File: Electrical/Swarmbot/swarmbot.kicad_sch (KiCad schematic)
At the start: 5 parts, among them J1 Conn_02x07_Counter_Clockwise, J2 Conn_02x07_Counter_Clockwise

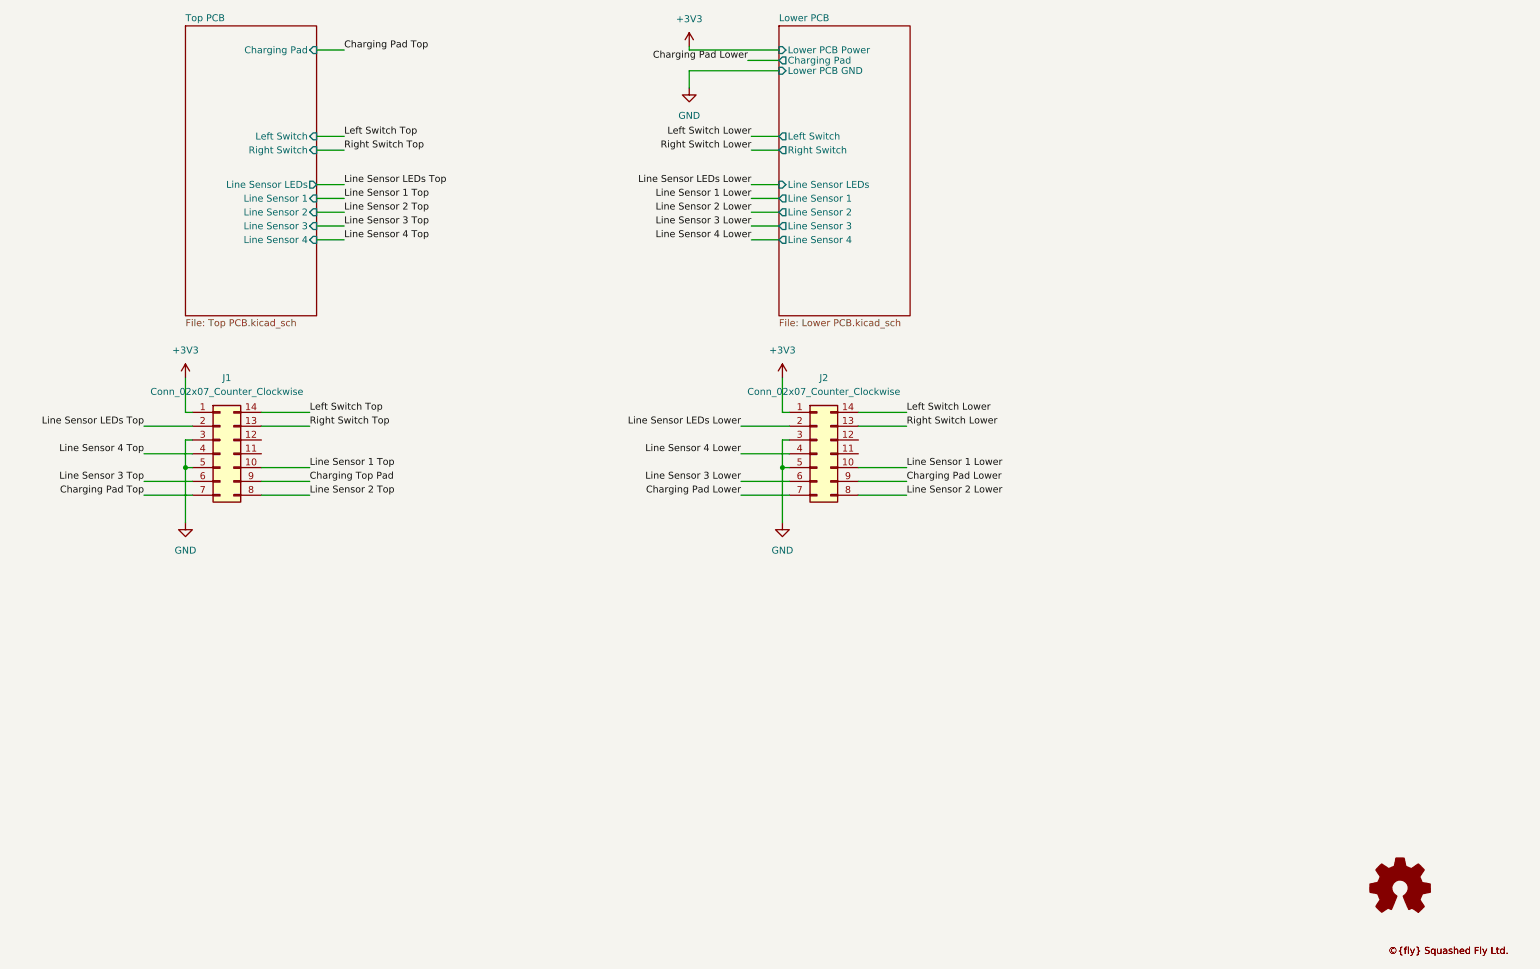
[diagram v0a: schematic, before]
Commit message: some little changes have been made
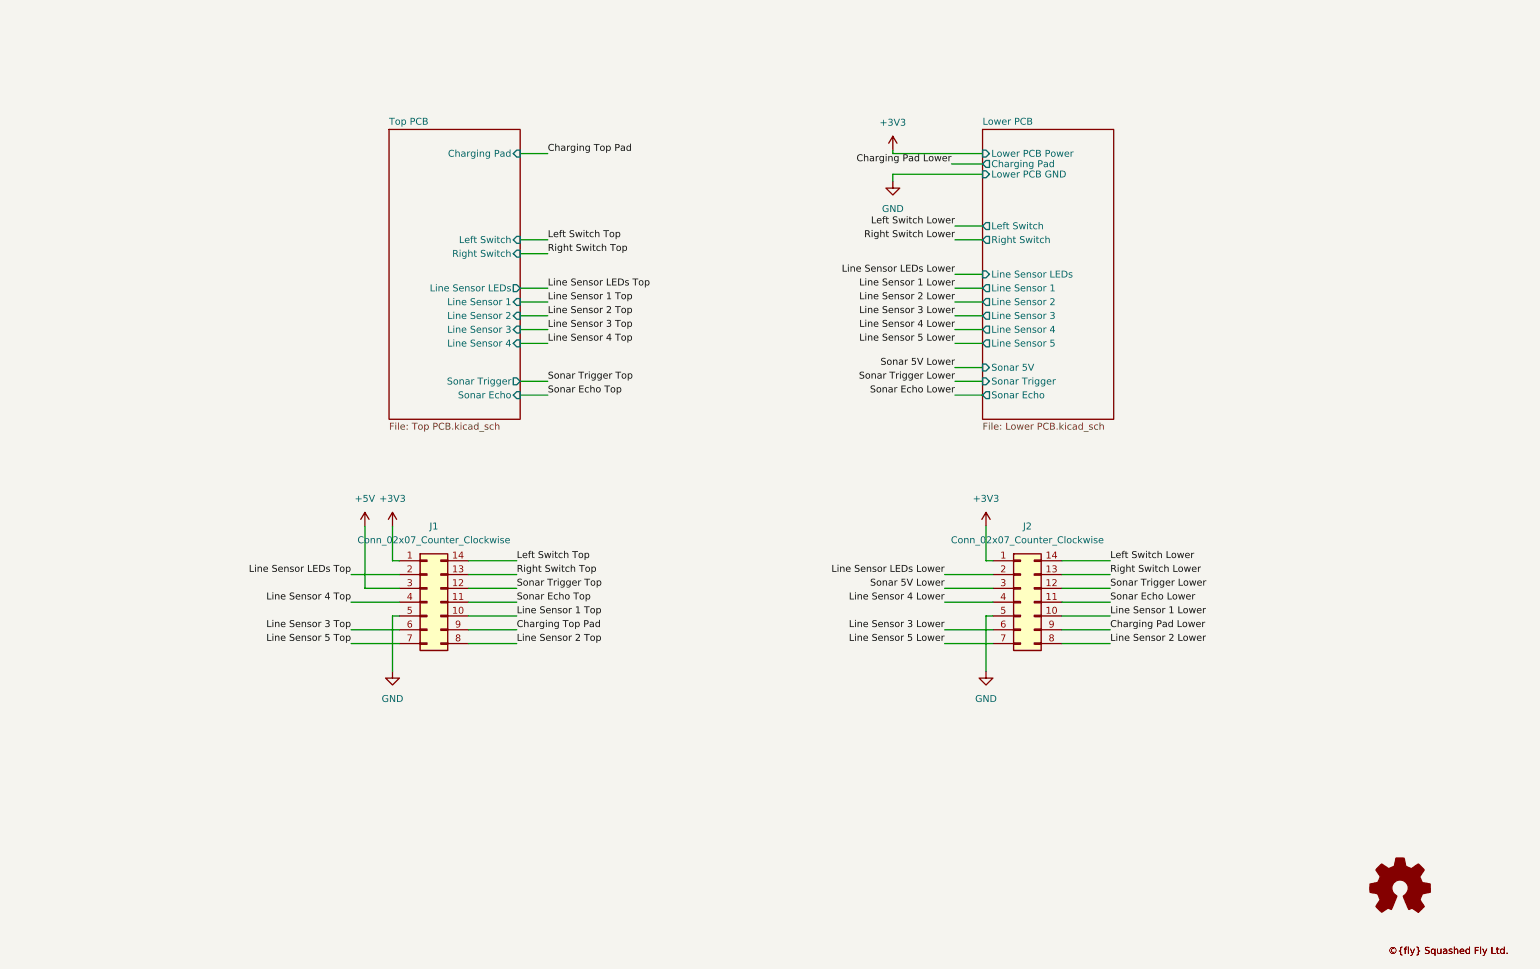
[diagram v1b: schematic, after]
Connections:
- net Charging Pad Lower: no longer J2.7 (Pin_7)
- net GND: no longer J1.3 (Pin_3), J2.3 (Pin_3)
- net Sonar Echo Top: now reaches J1.11 (Pin_11)
- net Sonar Trigger Top: now reaches J1.12 (Pin_12)
- net Sonar Echo Lower: now reaches J2.11 (Pin_11)
- net Sonar Trigger Lower: now reaches J2.12 (Pin_12)
- net Charging Pad Top renamed Line Sensor 5 Top
- new net +5V: J1.3 (Pin_3)
- new net Line Sensor 5 Lower: J2.7 (Pin_7)
- new net Sonar 5V Lower: J2.3 (Pin_3)
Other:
- sheet Lower PCB ports: added Line Sensor 5, Sonar 5V, Sonar Echo, Sonar Trigger; removed none
- sheet Top PCB ports: added Sonar Echo, Sonar Trigger; removed none
- moved on the sheet: J1, J2

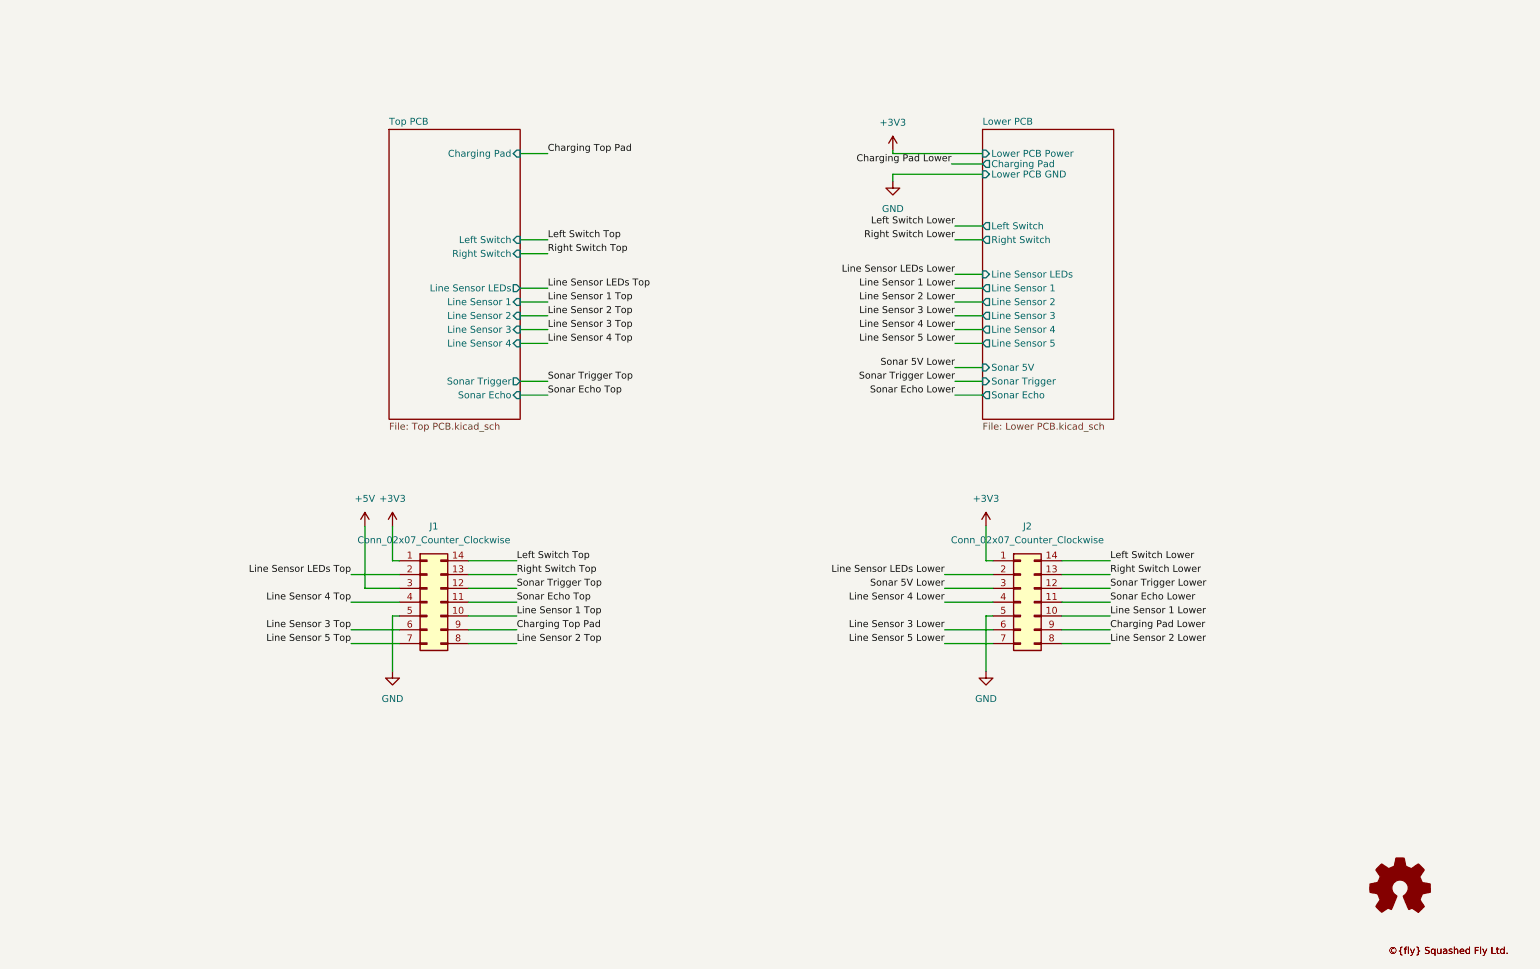
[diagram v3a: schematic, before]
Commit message: Made some Changes
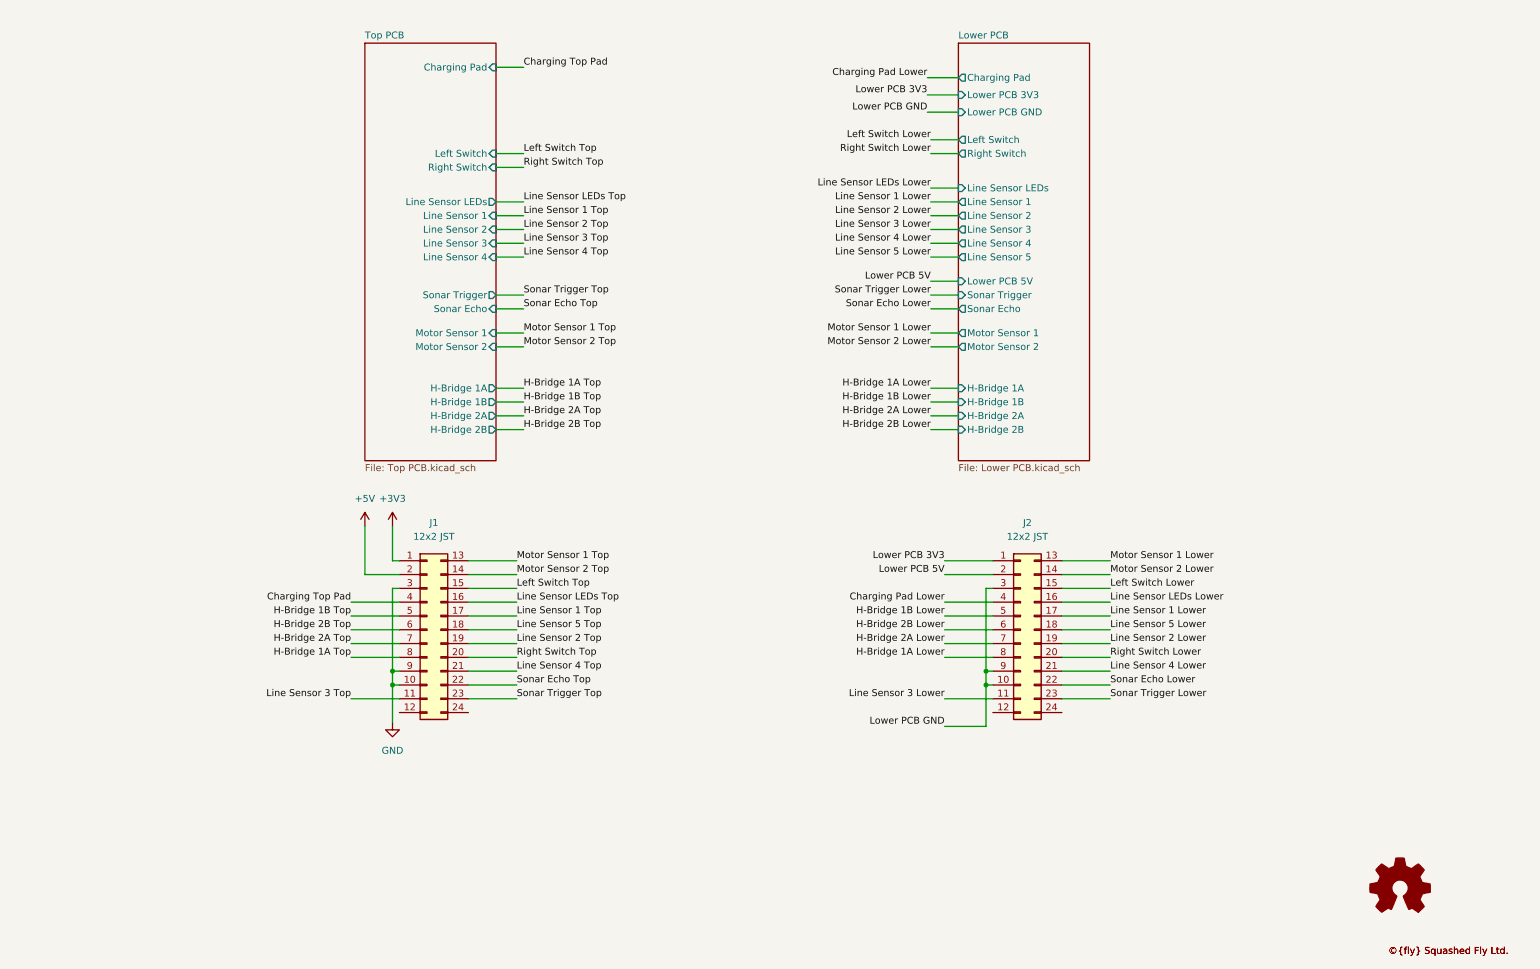
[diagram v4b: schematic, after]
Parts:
- removed J1, J2: Conn_02x07_Counter_Clockwise, Connector_JST:JST_PUD_B14B-PUDSS_2x07_P2.00mm_Vertical, symbol Connector_Generic:Conn_02x07_Counter_Clockwise
- added J1, J2: 12x2 JST, Connector_JST:JST_PUD_B24B-PUDSS_2x12_P2.00mm_Vertical, symbol Connector_Generic:Conn_02x12_Top_Bottom
- Logo2: footprint SquashedFly Logo:SquashedFlyBrightCopper -> SquashedFly Logo:SquashedFlySilk
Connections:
- net +3V3: now also J1.1 (Pin_1)
- net +5V: now also J1.2 (Pin_2)
- net Charging Pad Lower: now also J2.4 (Pin_4)
- net Charging Top Pad: now also J1.4 (Pin_4)
- net GND: now also J1.10 (Pin_10), J1.3 (Pin_3), J1.9 (Pin_9)
- net Left Switch Lower: now also J2.15 (Pin_15)
- net Left Switch Top: now also J1.15 (Pin_15)
- net Line Sensor 1 Lower: now also J2.17 (Pin_17)
- net Line Sensor 1 Top: now also J1.17 (Pin_17)
- net Line Sensor 2 Lower: now also J2.19 (Pin_19)
- net Line Sensor 2 Top: now also J1.19 (Pin_19)
- net Line Sensor 3 Lower: now also J2.11 (Pin_11)
- net Line Sensor 3 Top: now also J1.11 (Pin_11)
- net Line Sensor 4 Lower: now also J2.21 (Pin_21)
- net Line Sensor 4 Top: now also J1.21 (Pin_21)
- net Line Sensor 5 Lower: now also J2.18 (Pin_18)
- net Line Sensor 5 Top: now also J1.18 (Pin_18)
- net Line Sensor LEDs Lower: now also J2.16 (Pin_16)
- net Line Sensor LEDs Top: now also J1.16 (Pin_16)
- net Right Switch Lower: now also J2.20 (Pin_20)
- net Right Switch Top: now also J1.20 (Pin_20)
- net Sonar Echo Lower: now also J2.22 (Pin_22)
- net Sonar Echo Top: now also J1.22 (Pin_22)
- net Sonar Trigger Lower: now also J2.23 (Pin_23)
- net Sonar Trigger Top: now also J1.23 (Pin_23)
- new net H-Bridge 1A Lower: J2.8 (Pin_8)
- new net H-Bridge 1A Top: J1.8 (Pin_8)
- new net H-Bridge 1B Lower: J2.5 (Pin_5)
- new net H-Bridge 1B Top: J1.5 (Pin_5)
- new net H-Bridge 2A Lower: J2.7 (Pin_7)
- new net H-Bridge 2A Top: J1.7 (Pin_7)
- new net H-Bridge 2B Lower: J2.6 (Pin_6)
- new net H-Bridge 2B Top: J1.6 (Pin_6)
- new net Lower PCB 3V3: J2.1 (Pin_1)
- new net Lower PCB 5V: J2.2 (Pin_2)
- new net Lower PCB GND: J2.10 (Pin_10), J2.3 (Pin_3), J2.9 (Pin_9)
- new net Motor Sensor 1 Lower: J2.13 (Pin_13)
- new net Motor Sensor 1 Top: J1.13 (Pin_13)
- new net Motor Sensor 2 Lower: J2.14 (Pin_14)
- new net Motor Sensor 2 Top: J1.14 (Pin_14)
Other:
- sheet Lower PCB ports: added H-Bridge 1A, H-Bridge 1B, H-Bridge 2A, H-Bridge 2B, Lower PCB 3V3, Lower PCB 5V, Motor Sensor 1, Motor Sensor 2; removed Lower PCB Power, Sonar 5V
- sheet Top PCB ports: added H-Bridge 1A, H-Bridge 1B, H-Bridge 2A, H-Bridge 2B, Motor Sensor 1, Motor Sensor 2; removed none
